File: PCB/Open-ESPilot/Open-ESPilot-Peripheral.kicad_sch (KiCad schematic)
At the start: 58 parts, among them J10 UART1, J11 UART2, J12 I2C, J14 LED out, J5 PWM output, J6 RC in, J7 Vx, J8 GND, J9 UART0, M2 GY91, Q2 BC847, Q3 BC847, U5 Micro_SD_Card

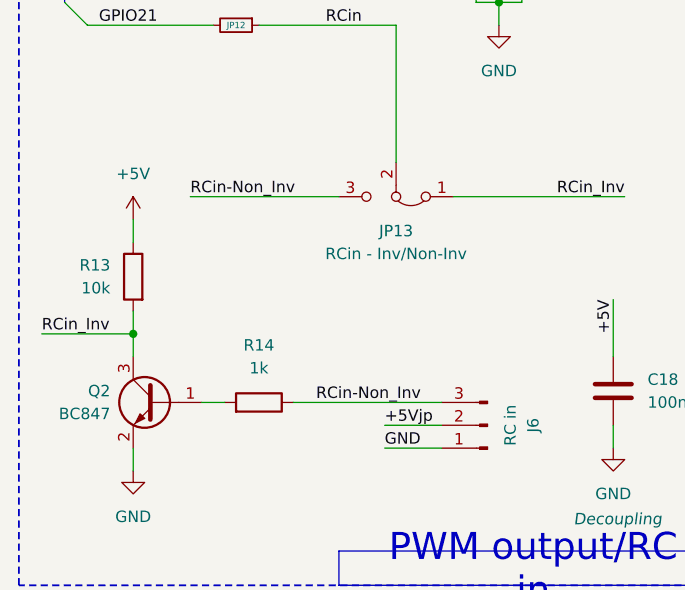
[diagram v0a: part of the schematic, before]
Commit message: I'm rushing it! :( Finished the PCB
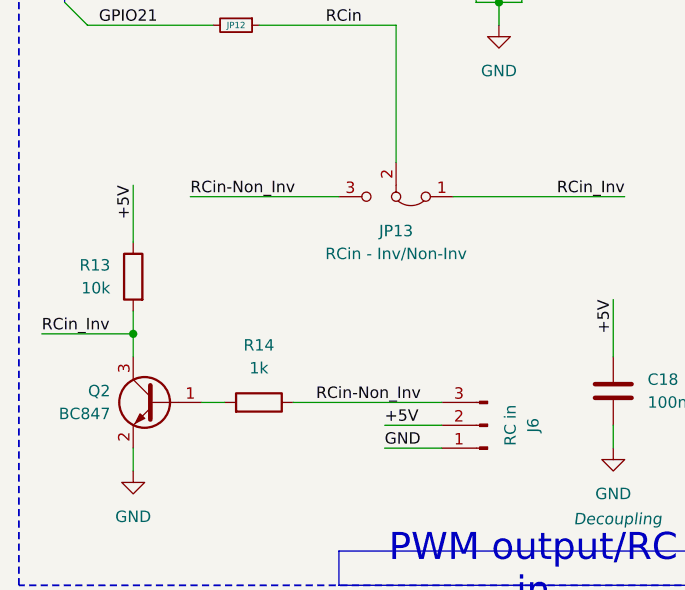
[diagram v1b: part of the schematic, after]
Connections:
- net +5V: now also J6.2 (Pin_2)
- net +5Vjp: no longer J6.2 (Pin_2)
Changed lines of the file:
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@@
 	(wire
 		(pts
+			(xy 29.21 148.59) (xy 29.21 154.94)
+		)
+		(stroke
+			(width 0)
+			(type default)
+		)
+	)
+	(wire
+		(pts
 			(xy 254 74.93) (xy 254 76.2)
 		)
@@
 		)
 	)
-	(wire
-		(pts
-			(xy 29.21 152.4) (xy 29.21 154.94)
-		)
-		(stroke
-			(width 0)
-			(type default)
-		)
-	)
 	(bus
 		(pts
@@
 		)
 	)
-	(label "+5Vjp"
+	(label "+5V"
 		(at 57.15 175.26 0)
 		(effects
@@
 		)
 	)
+	(label "+5V"
+		(at 29.21 148.59 270)
+		(effects
+			(font
+				(size 1.27 1.27)
+			)
+			(justify right bottom)
+		)
+	)
 	(label "BUZZER"
 		(at 229.87 82.55 180)
@@
 					(unit 1)
 				)
-			)
-		)
-	)
-	(symbol
-		(lib_id "power:+5V")
-		(at 29.21 152.4 0)
-		(mirror y)
-		(unit 1)
-		(exclude_from_sim no)
-		(in_bom yes)
-		(on_board yes)
-		(dnp no)
-		(property "Reference" "#PWR041"
-			(at 29.21 156.21 0)
-			(effects
-				(font
-					(size 1.27 1.27)
-				)
-				(hide yes)
-			)
-		)
-		(property "Value" "+5V"
-			(at 29.21 147.32 0)
-			(effects
-				(font
-					(size 1.27 1.27)
-				)
-			)
-		)
-		(property "Footprint" ""
-			(at 29.21 152.4 0)
-			(effects
-				(font
-					(size 1.27 1.27)
-				)
-				(hide yes)
-			)
-		)
-		(property "Datasheet" ""
-			(at 29.21 152.4 0)
-			(effects
-				(font
-					(size 1.27 1.27)
-				)
-				(hide yes)
-			)
-		)
-		(property "Description" "Power symbol creates a global label with name \"+5V\""
-			(at 29.21 152.4 0)
-			(effects
-				(font
-					(size 1.27 1.27)
-				)
-				(hide yes)
-			)
-		)
-		(pin "1"
-		)
-		(instances
-			(project "Open-ESPilot"
-				(path "/2992e60d-a645-4cd7-90ae-fe72311b6bee/e6a81ea1-6816-412d-a6dc-b491c7035238"
-					(reference "#PWR041")
-					(unit 1)
-				)
